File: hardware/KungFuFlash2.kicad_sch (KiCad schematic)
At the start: 52 parts, among them J1 SWD, J2 USB_B_Micro, J3 Wifi, Q1 BC817, SW1 Reset, SW2 Menu, SW3 Special, U1 C64-Exp-Port, U2 AMS1117-3.3, U3 STM32H7B0VBTx, Y1 25MHz

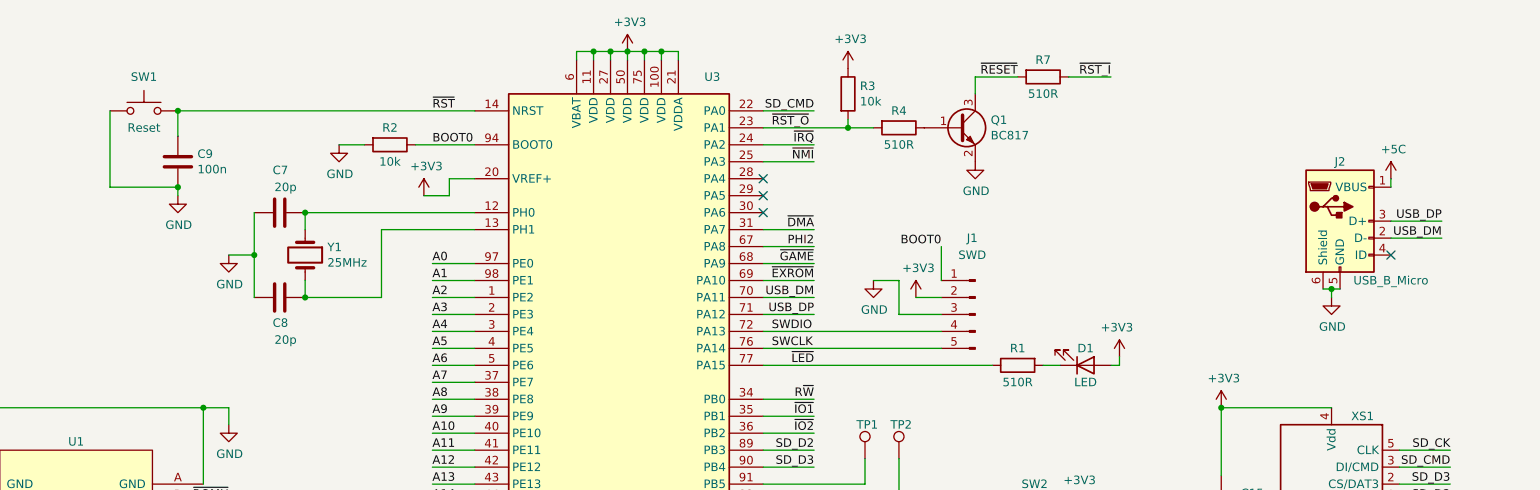
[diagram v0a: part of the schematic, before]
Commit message: Add USB C and JLCPCB files
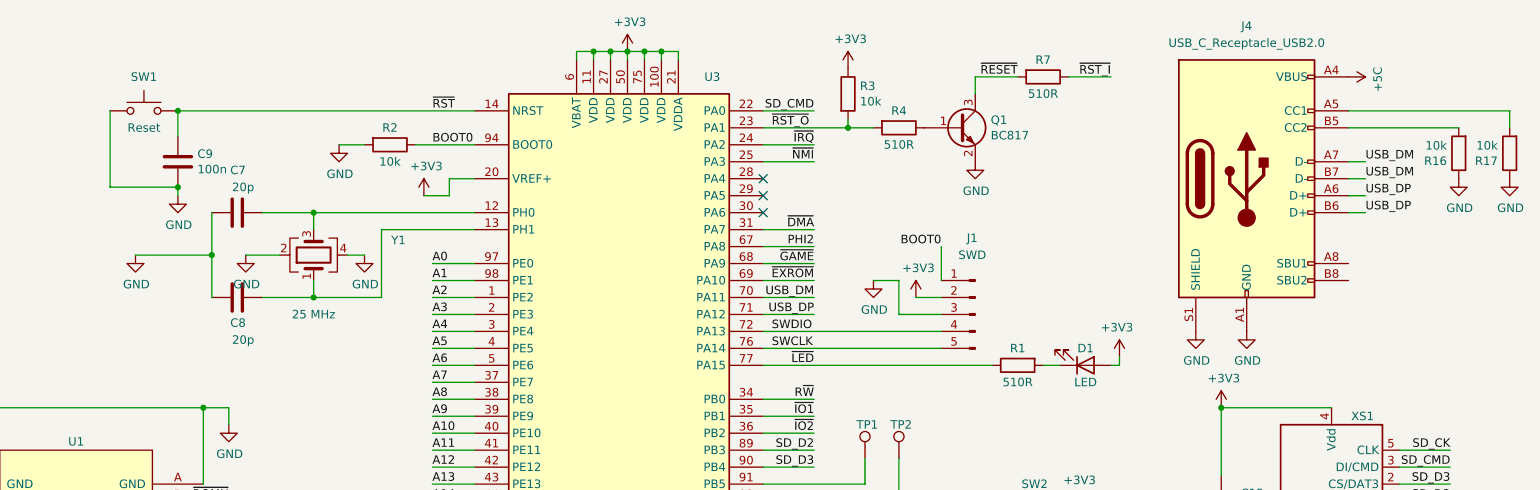
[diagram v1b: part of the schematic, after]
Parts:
- removed J2: USB_B_Micro, KungFuFlash2:Conn_USBmicro-B_ebay-side_TH, symbol KungFuFlash2:USB_B_Micro-Connector
- removed Y1: 25MHz, Crystal:Crystal_SMD_5032-2Pin_5.0x3.2mm, symbol Device:Crystal
- added J4: USB_C_Receptacle_USB2.0, Connector_USB:USB_C_Receptacle_XKB_U262-16XN-4BVC11, symbol Connector:USB_C_Receptacle_USB2.0
- added R16, R17: 10k, Resistor_SMD:R_0805_2012Metric_Pad1.20x1.40mm_HandSolder, symbol Device:R
- added Y1: 25 MHz, Crystal:Crystal_SMD_3225-4Pin_3.2x2.5mm, symbol Device:Crystal_GND24
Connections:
- net +5C: now also J4.A4 (VBUS), J4.A9 (VBUS), J4.B4 (VBUS), J4.B9 (VBUS)
- net GND: now also J4.A1 (GND), J4.A12 (GND), J4.B1 (GND), J4.B12 (GND), J4.S1 (SHIELD), R16.1, R17.1, Y1.2, Y1.4
- net USB_DM: now also J4.A7 (D-), J4.B7 (D-)
- net USB_DP: now also J4.A6 (D+), J4.B6 (D+)
- net at C7.2, U3.12 (PH0): now also Y1.3
- net at C8.2, U3.13 (PH1): now also Y1.1
- new net: J4.B5 (CC2), R16.2
- new net: J4.A5 (CC1), R17.2
- no-connect marks 26 -> 25
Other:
- moved on the sheet: C7, C8
